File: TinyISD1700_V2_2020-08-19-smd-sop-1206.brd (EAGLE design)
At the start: 38.1 x 48.3 mm, 18 parts, among them IC3 LM317MDT, U1 ATTINY4313-SU

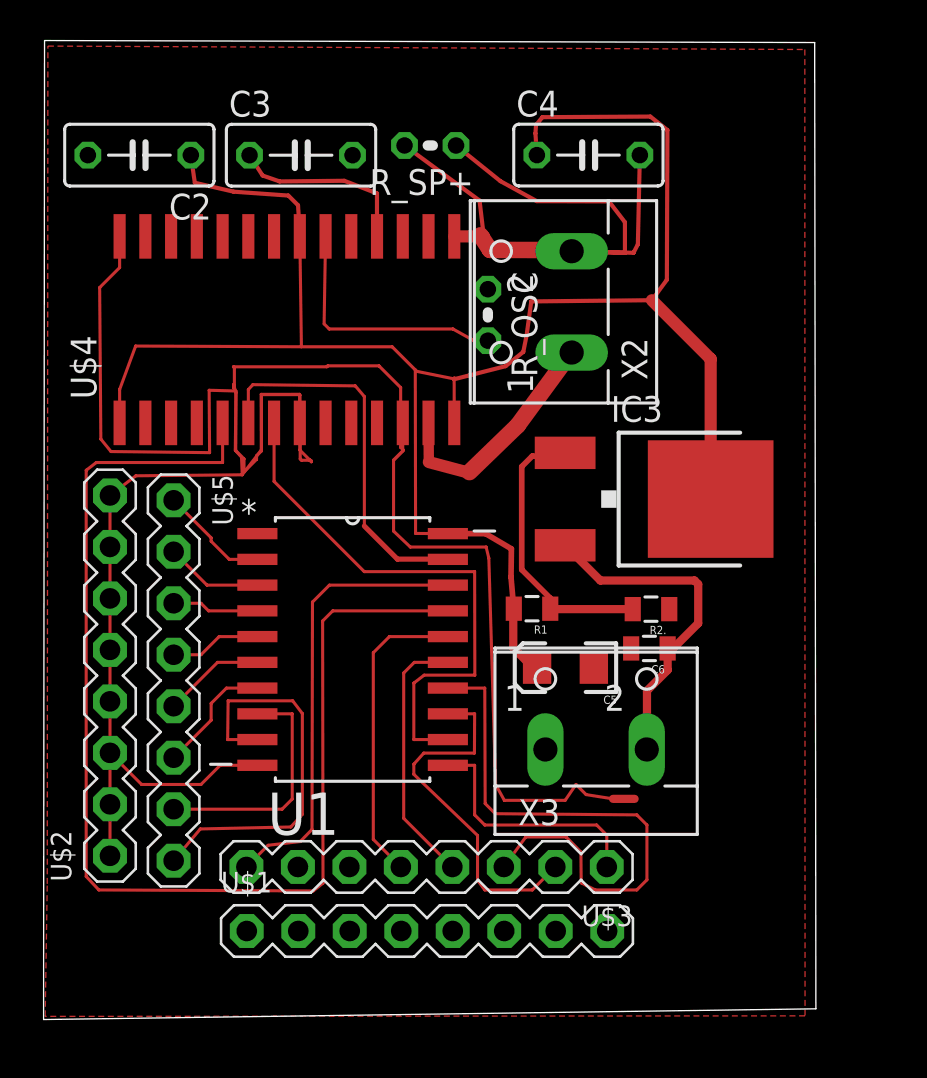
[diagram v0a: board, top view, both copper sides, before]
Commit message: commit
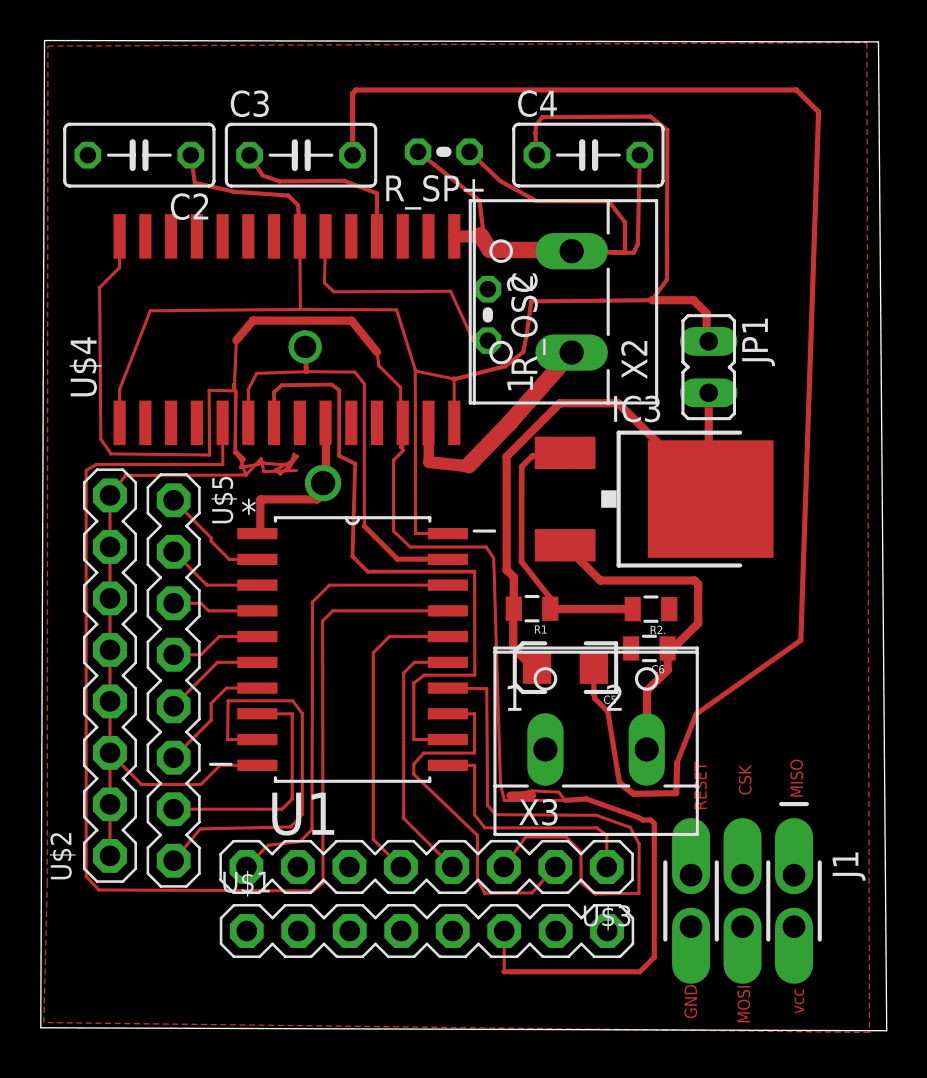
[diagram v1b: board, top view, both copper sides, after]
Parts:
- added J1: AVR_SPI_PRG_6OFFSET_PADS, SparkFun:2X3_OFFSET
- added JP1: (no value), jumper:JP1
- moved R_SP+ 0.74 mm to (17.8, 39.6)
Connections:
- new net ANALN: J1.5, U$4.9, U1.1
- new net MISO: J1.1
- new net N$19: C5.A, IC3.4, JP1.2, R1.2
- net CSK: now also J1.3
- net GND: now also J1.6
- net MOSI: now also J1.4
- net VCC: now also J1.2, JP1.1; no longer C5.A, IC3.4, R1.2
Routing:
- net GND: track 125.7 -> 213.6 mm
- net N$19: track 0.00 -> 29.4 mm
- net VCC: track 95.9 -> 80.5 mm
- net ANALN: track 0.00 -> 8.61 mm
- net SS: track 27.3 -> 32.7 mm
- net CSK: track 18.9 -> 21.1 mm
- net N$3: track 28.5 -> 27.8 mm
- net N$7: track 13.0 -> 12.3 mm
- net N$4: track 21.8 -> 21.1 mm
- net N$1: track 12.6 -> 12.1 mm
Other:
- board size 38.1 x 48.3 mm -> 41.7 x 48.9 mm
- board text added: "CSK"
- board text added: "GND"
- board text added: "MISO"
- board text added: "MOSI"
- board text added: "RESET"
- board text added: "vcc"
